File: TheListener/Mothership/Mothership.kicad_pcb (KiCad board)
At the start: 2 copper layers, 65 parts, among them J1 RJ45, J2 RJ45, J3 RJ45, J4 RJ45, J5 RJ45, J6 RJ45, J7 RJ45, J8 RJ45, J9 Conn_01x02_Female, U1 SP3491, U10 AMS1117-3.3, U11 NID35-5, U12 Teensy3.5, U2 SP3491, U3 SP3491, U4 SP3491, U5 SP3491, U6 SP3491, U7 SP3491, U8 SP3491, U9 AMS1117-3.3

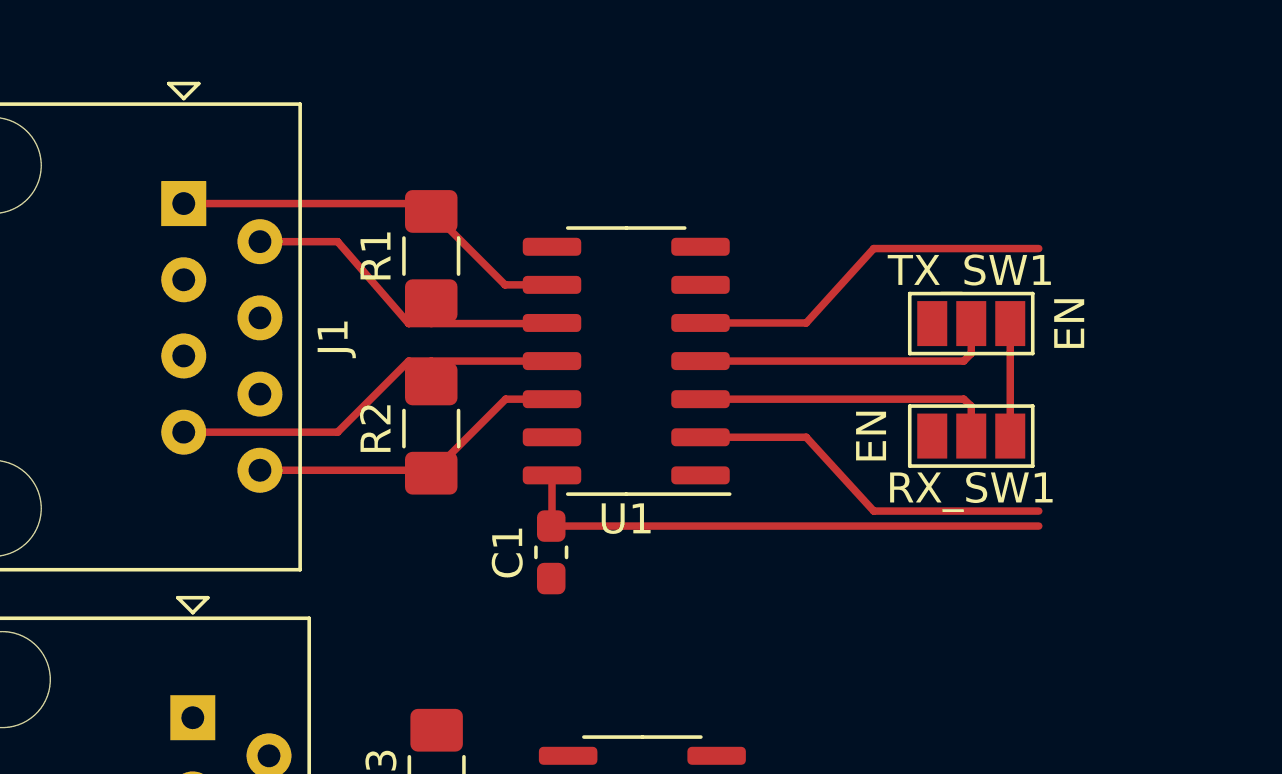
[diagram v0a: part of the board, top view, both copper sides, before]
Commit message: updates to layout
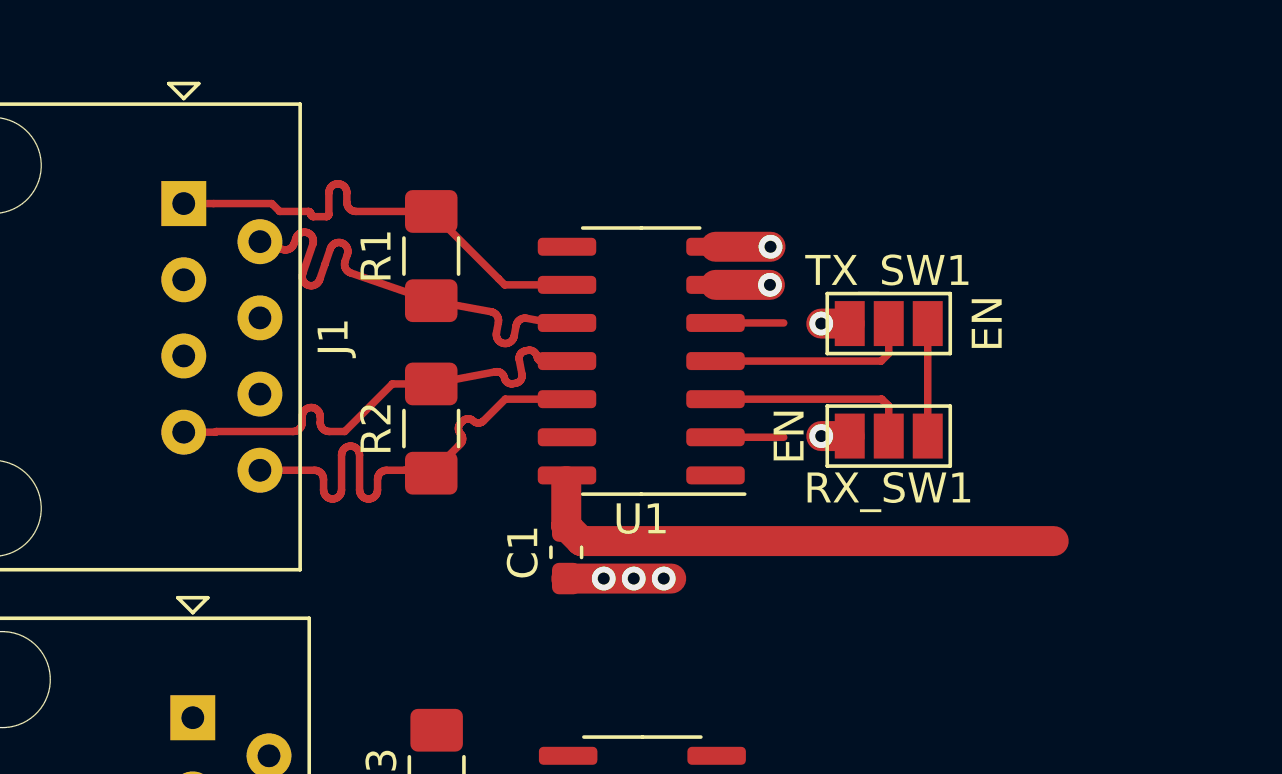
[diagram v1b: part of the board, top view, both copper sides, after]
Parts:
- moved RX_SW1 2.75 mm to (58.2, 47.0)
- moved TX_SW1 2.75 mm to (58.2, 43.2)
- moved C1 0.50 mm to (47.5, 50.9)
- moved U1 0.50 mm to (50.0, 44.5)
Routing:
- net T_1: track 12.4 -> 2.27 mm
- net R_1: track 12.4 -> 2.27 mm
- net GND: track 0.00 -> 9.05 mm, vias 0 -> 7
- net Net-(J1-Pad8): track 10.3 -> 15.6 mm
- net Net-(TX_SW1-Pad2): track 10.1 -> 6.88 mm
- net Net-(J1-Pad2): track 12.3 -> 15.5 mm
- net Net-(RX_SW1-Pad2): track 10.1 -> 7.21 mm
- net Net-(J1-Pad1): track 13.0 -> 15.6 mm
- net Net-(J1-Pad7): track 14.0 -> 15.4 mm
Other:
- net class Default: clearance 0.2 -> 0.25
- net class High Current added: clearance 0.5, trace_width 5, via_dia 1.6, via_drill 0.8
- net class Low Current added: clearance 0.25, trace_width 1, via_dia 0.8, via_drill 0.4
- rule pad_to_mask_clearance: 0.051 -> 0.05
- rule trace_clearance: 0.2 -> 0.25
- rule via_min_size: 0.4 -> 0.6
